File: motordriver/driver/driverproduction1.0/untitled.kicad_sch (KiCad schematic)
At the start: 34 parts, among them T230:? Transformer_1P_1S

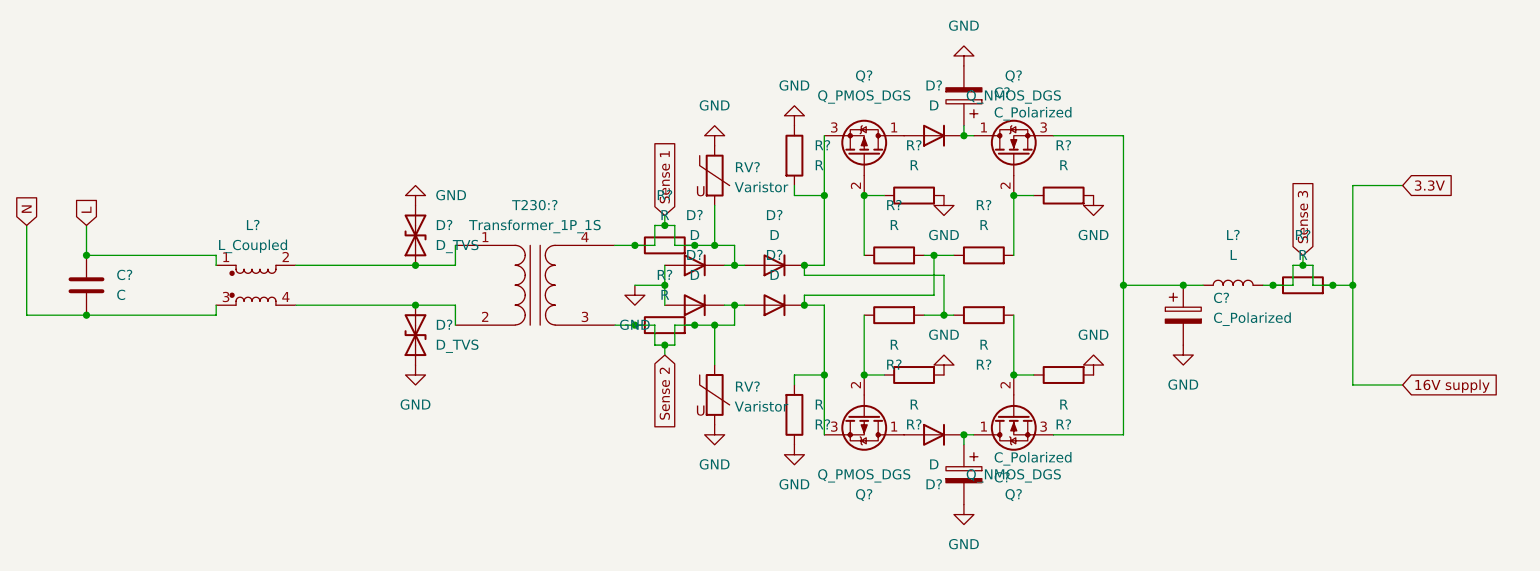
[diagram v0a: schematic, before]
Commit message: 3 hours
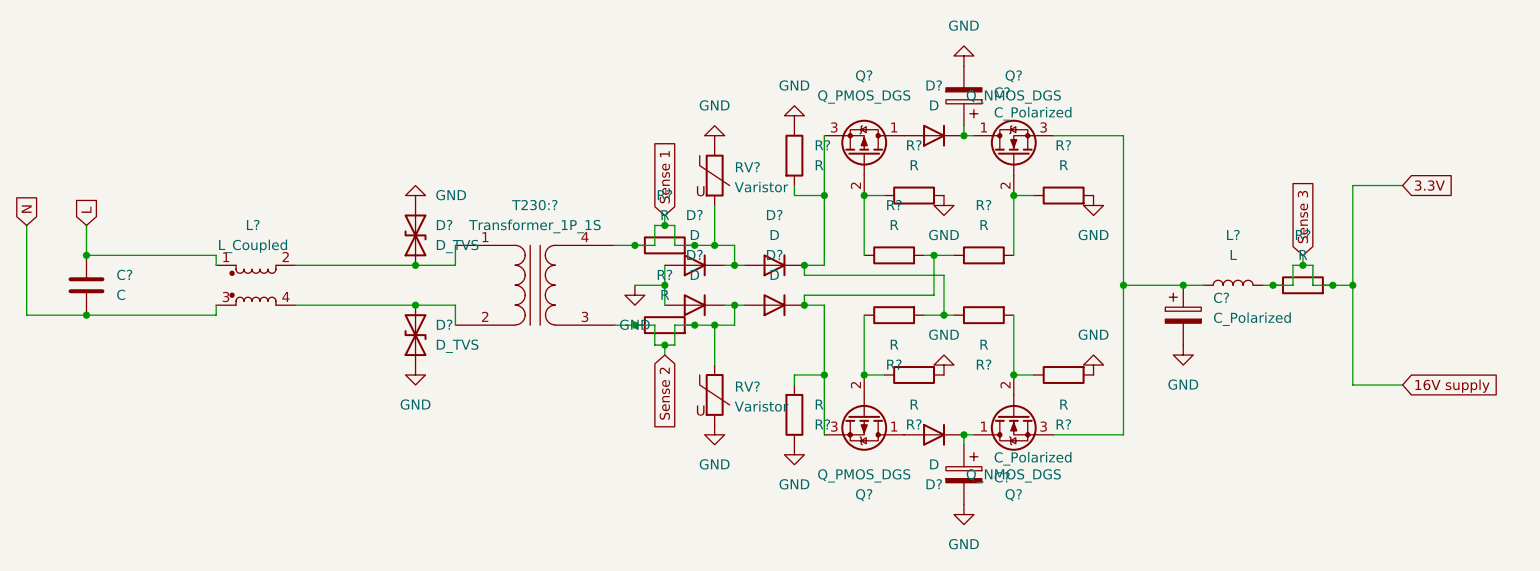
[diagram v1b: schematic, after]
